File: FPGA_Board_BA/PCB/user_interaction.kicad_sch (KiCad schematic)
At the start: 15 parts, among them SW1 TL3305BF100QG, SW2 TL3305BF100QG

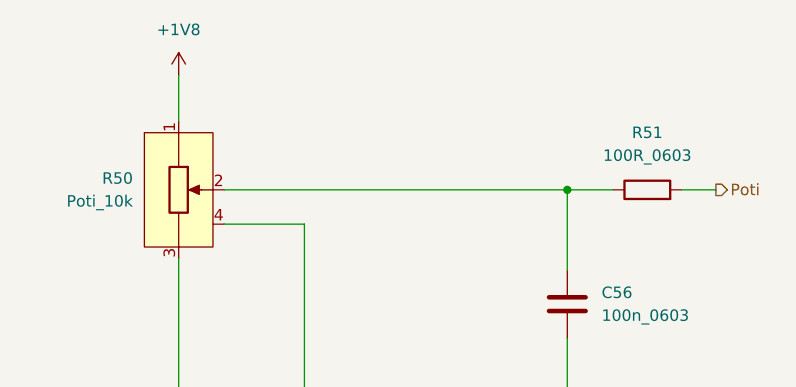
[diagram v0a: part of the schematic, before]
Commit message: Besprechung mit Leo
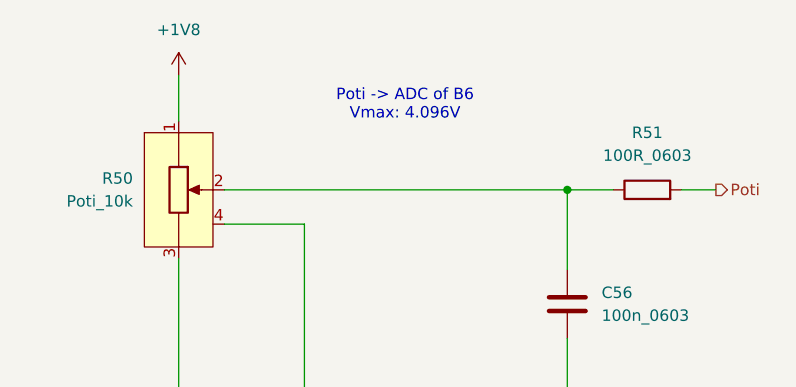
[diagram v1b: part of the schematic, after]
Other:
- note added: "Poti -> ADC of B6 Vmax: 4.096V"
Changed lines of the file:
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@@
 	(generator_version "9.0")
 	(paper "A4")
+	(text "Poti -> ADC of B6\nVmax: 4.096V"
+		(exclude_from_sim no)
+		(at 216.916 57.912 0)
+		(effects
+			(font
+				(size 1.27 1.27)
+			)
+		)
+	)
 	(junction
 		(at 133.35 139.7)
